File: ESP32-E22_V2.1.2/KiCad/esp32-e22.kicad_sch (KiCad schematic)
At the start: 46 parts, among them J1 Conn_01x02_Socket, J10 Conn_01x02_Socket, J11 Conn_01x04_Socket, J12 Conn_01x02_Socket, J3 Screw_Terminal_01x02, J4 Conn_01x04_Socket, J5 Conn_01x03_Socket, J6 Conn_01x04_Socket, J7 Conn_01x05_Socket, J8 SMA, J9 Conn_01x02_Socket, SW1 SW_Push, U1 ESP32-DevKitC V4, U2 DM-OLED096-636, U3 E22-400M33S, U4 HW-613

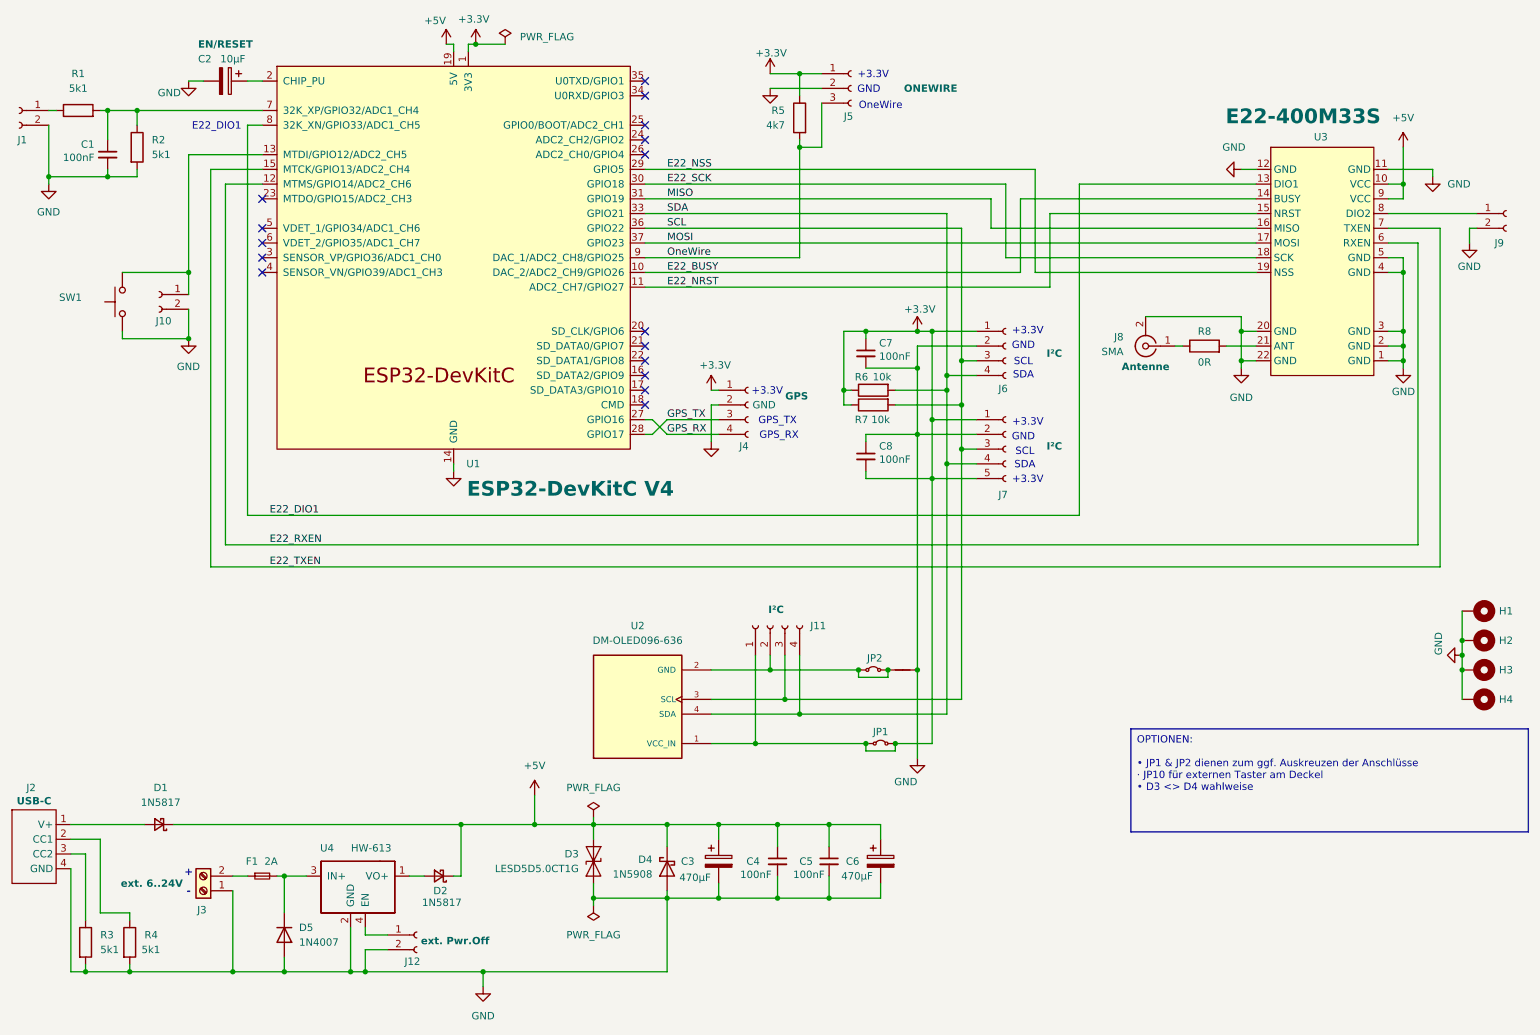
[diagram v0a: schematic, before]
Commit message: update
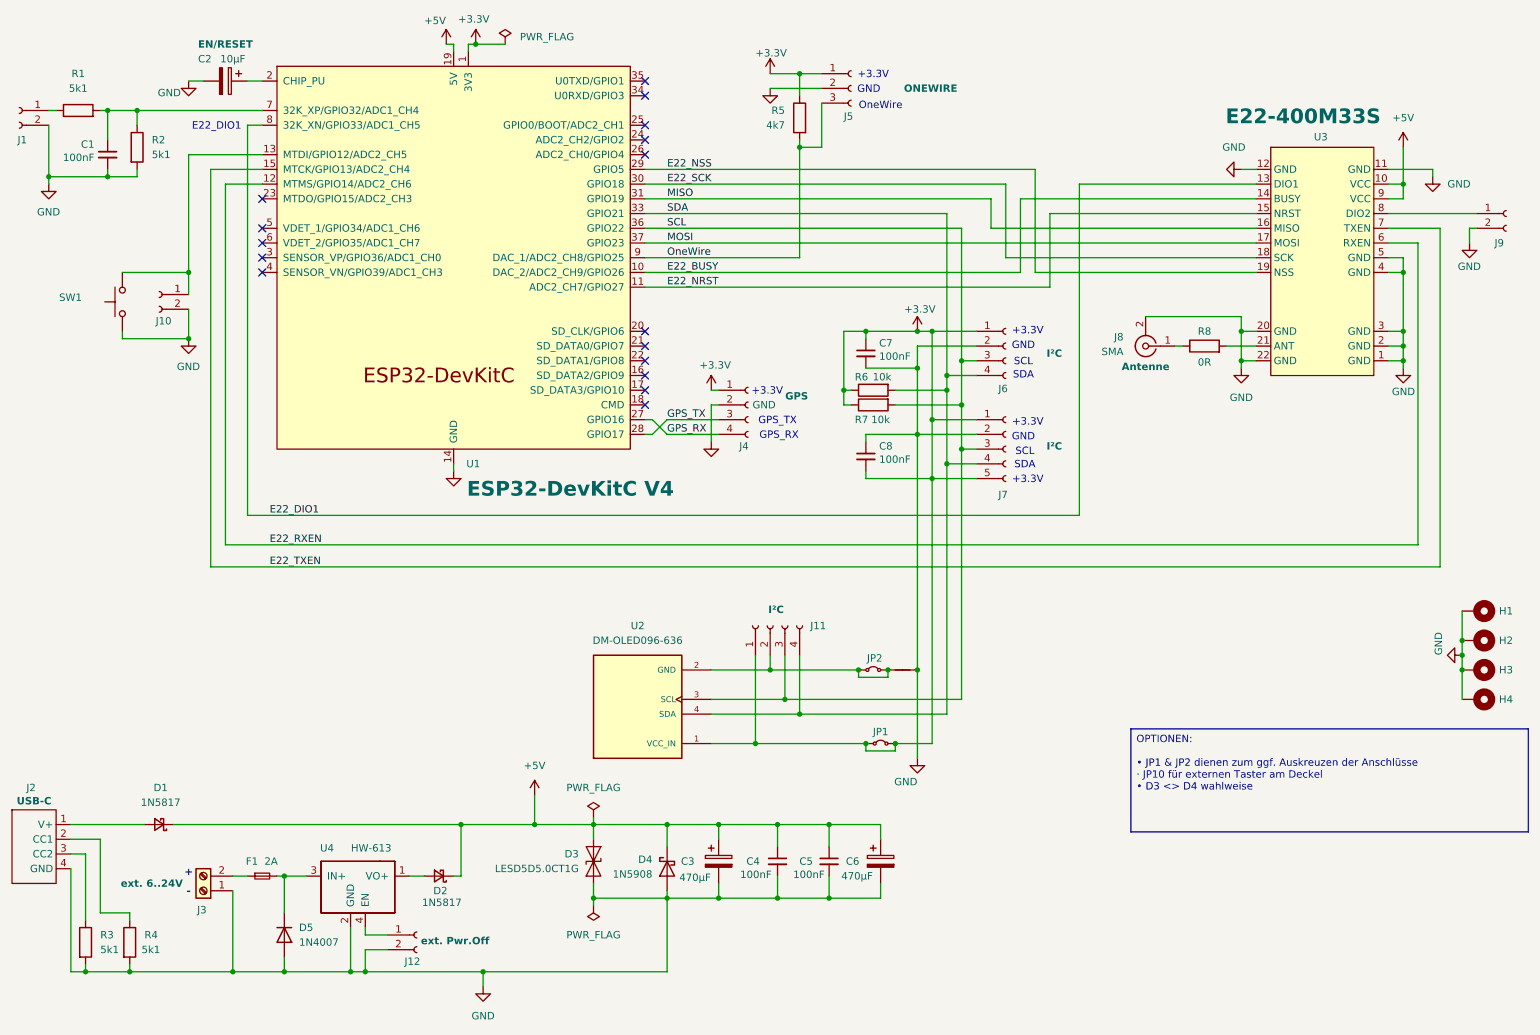
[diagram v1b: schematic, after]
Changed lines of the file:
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@@
 (kicad_sch
-	(version 20231120)
+	(version 20250114)
 	(generator "eeschema")
-	(generator_version "8.0")
+	(generator_version "9.0")
 	(paper "A4")
 	(title_block
@@
 		(company "OE3WAS")
 	)
+	(text "GND"
+		(exclude_from_sim no)
+		(at 193.548 94.488 0)
+		(effects
+			(font
+				(size 1.27 1.27)
+			)
+		)
+	)
+	(text "SCL"
+		(exclude_from_sim no)
+		(at 193.548 81.534 0)
+		(effects
+			(font
+				(size 1.27 1.27)
+			)
+		)
+	)
+	(text "GND"
+		(exclude_from_sim no)
+		(at 193.548 78.74 0)
+		(effects
+			(font
+				(size 1.27 1.27)
+			)
+		)
+	)
+	(text "SCL"
+		(exclude_from_sim no)
+		(at 193.802 97.028 0)
+		(effects
+			(font
+				(size 1.27 1.27)
+			)
+		)
+	)
+	(text "+3.3V"
+		(exclude_from_sim no)
+		(at 149.352 86.614 0)
+		(effects
+			(font
+				(size 1.27 1.27)
+			)
+		)
+	)
+	(text "+3.3V"
+		(exclude_from_sim no)
+		(at 194.31 101.854 0)
+		(effects
+			(font
+				(size 1.27 1.27)
+			)
+		)
+	)
+	(text "GND"
+		(exclude_from_sim no)
+		(at 166.878 34.544 0)
+		(effects
+			(font
+				(size 1.27 1.27)
+			)
+		)
+	)
+	(text "-"
+		(exclude_from_sim no)
+		(at 49.53 172.974 0)
+		(effects
+			(font
+				(size 1.27 1.27)
+				(thickness 0.254)
+				(bold yes)
+			)
+		)
+	)
+	(text "GPS_TX"
+		(exclude_from_sim no)
+		(at 151.13 91.694 0)
+		(effects
+			(font
+				(size 1.27 1.27)
+			)
+		)
+	)
+	(text "OneWire"
+		(exclude_from_sim no)
+		(at 168.91 37.338 0)
+		(effects
+			(font
+				(size 1.27 1.27)
+			)
+		)
+	)
+	(text "SDA"
+		(exclude_from_sim no)
+		(at 193.802 99.314 0)
+		(effects
+			(font
+				(size 1.27 1.27)
+			)
+		)
+	)
+	(text "SDA"
+		(exclude_from_sim no)
+		(at 193.548 83.82 0)
+		(effects
+			(font
+				(size 1.27 1.27)
+			)
+		)
+	)
+	(text "+3.3V"
+		(exclude_from_sim no)
+		(at 194.31 76.2 0)
+		(effects
+			(font
+				(size 1.27 1.27)
+			)
+		)
+	)
+	(text "+"
+		(exclude_from_sim no)
+		(at 49.53 169.672 0)
+		(effects
+			(font
+				(size 1.27 1.27)
+				(thickness 0.254)
+				(bold yes)
+			)
+		)
+	)
+	(text "GPS_RX"
+		(exclude_from_sim no)
+		(at 151.384 94.234 0)
+		(effects
+			(font
+				(size 1.27 1.27)
+			)
+		)
+	)
+	(text "+3.3V"
+		(exclude_from_sim no)
+		(at 194.31 91.948 0)
+		(effects
+			(font
+				(size 1.27 1.27)
+			)
+		)
+	)
+	(text "E22_DIO1"
+		(exclude_from_sim no)
+		(at 54.356 40.894 0)
+		(effects
+			(font
+				(size 1.27 1.27)
+			)
+		)
+	)
+	(text "+3.3V"
+		(exclude_from_sim no)
+		(at 167.64 32.004 0)
+		(effects
+			(font
+				(size 1.27 1.27)
+			)
+		)
+	)
+	(text_box "OPTIONEN:\n\n• JP1 & JP2 dienen zum ggf. Auskreuzen der Anschlüsse\n· JP10 für externen Taster am Deckel\n• D3 <> D4 wahlweise\n\n"
+		(exclude_from_sim yes)
+		(at 212.09 144.78 0)
+		(size 68.58 17.78)
+		(margins 0.9525 0.9525 0.9525 0.9525)
+		(stroke
+			(width 0)
+			(type default)
+		)
+		(fill
+			(type none)
+		)
+		(effects
+			(font
+				(size 1.27 1.27)
+			)
+			(justify left top)
+		)
+	)
 	(junction
 		(at 166.37 76.2)
@@
 		)
 	)
-	(text_box "OPTIONEN:\n\n• JP1 & JP2 dienen zum ggf. Auskreuzen der Anschlüsse\n· JP10 für externen Taster am Deckel\n• D3 <> D4 wahlweise\n\n"
-		(exclude_from_sim yes)
-		(at 212.09 144.78 0)
-		(size 68.58 17.78)
-		(stroke
-			(width 0)
-			(type default)
-		)
-		(fill
-			(type none)
-		)
-		(effects
-			(font
-				(size 1.27 1.27)
-			)
-			(justify left top)
-		)
-	)
-	(text "GND"
-		(exclude_from_sim no)
-		(at 193.548 94.488 0)
-		(effects
-			(font
-				(size 1.27 1.27)
-			)
-		)
-	)
-	(text "SCL"
-		(exclude_from_sim no)
-		(at 193.548 81.534 0)
-		(effects
-			(font
-				(size 1.27 1.27)
-			)
-		)
-	)
-	(text "GND"
-		(exclude_from_sim no)
-		(at 193.548 78.74 0)
-		(effects
-			(font
-				(size 1.27 1.27)
-			)
-		)
-	)
-	(text "SCL"
-		(exclude_from_sim no)
-		(at 193.802 97.028 0)
-		(effects
-			(font
-				(size 1.27 1.27)
-			)
-		)
-	)
-	(text "+3.3V"
-		(exclude_from_sim no)
-		(at 149.352 86.614 0)
-		(effects
-			(font
-				(size 1.27 1.27)
-			)
-		)
-	)
-	(text "+3.3V"
-		(exclude_from_sim no)
-		(at 194.31 101.854 0)
-		(effects
-			(font
-				(size 1.27 1.27)
-			)
-		)
-	)
-	(text "GND"
-		(exclude_from_sim no)
-		(at 166.878 34.544 0)
-		(effects
-			(font
-				(size 1.27 1.27)
-			)
-		)
-	)
-	(text "-"
-		(exclude_from_sim no)
-		(at 49.53 172.974 0)
-		(effects
-			(font
-				(size 1.27 1.27)
-				(thickness 0.254)
-				(bold yes)
-			)
-		)
-	)
-	(text "GPS_TX"
-		(exclude_from_sim no)
-		(at 151.13 91.694 0)
-		(effects
-			(font
-				(size 1.27 1.27)
-			)
-		)
-	)
-	(text "OneWire"
-		(exclude_from_sim no)
-		(at 168.91 37.338 0)
-		(effects
-			(font
-				(size 1.27 1.27)
-			)
-		)
-	)
-	(text "SDA"
-		(exclude_from_sim no)
-		(at 193.802 99.314 0)
-		(effects
-			(font
-				(size 1.27 1.27)
-			)
-		)
-	)
-	(text "SDA"
-		(exclude_from_sim no)
-		(at 193.548 83.82 0)
-		(effects
-			(font
-				(size 1.27 1.27)
-			)
-		)
-	)
-	(text "+3.3V"
-		(exclude_from_sim no)
-		(at 194.31 76.2 0)
-		(effects
-			(font
-				(size 1.27 1.27)
-			)
-		)
-	)
-	(text "+"
-		(exclude_from_sim no)
-		(at 49.53 169.672 0)
-		(effects
-			(font
-				(size 1.27 1.27)
-				(thickness 0.254)
-				(bold yes)
-			)
-		)
-	)
-	(text "GPS_RX"
-		(exclude_from_sim no)
-		(at 151.384 94.234 0)
-		(effects
-			(font
-				(size 1.27 1.27)
-			)
-		)
-	)
-	(text "+3.3V"
-		(exclude_from_sim no)
-		(at 194.31 91.948 0)
-		(effects
-			(font
-				(size 1.27 1.27)
-			)
-		)
-	)
-	(text "E22_DIO1"
-		(exclude_from_sim no)
-		(at 54.356 40.894 0)
-		(effects
-			(font
-				(size 1.27 1.27)
-			)
-		)
-	)
-	(text "+3.3V"
-		(exclude_from_sim no)
-		(at 167.64 32.004 0)
-		(effects
-			(font
-				(size 1.27 1.27)
-			)
-		)
-	)
 	(label "E22_NRST"
 		(at 132.08 68.58 0)
-		(fields_autoplaced yes)
 		(effects
 			(font
@@
 	(label "SCL"
 		(at 132.08 58.42 0)
-		(fields_autoplaced yes)
 		(effects
 			(font
@@
 	(label "E22_BUSY"
 		(at 132.08 66.04 0)
-		(fields_autoplaced yes)
 		(effects
 			(font
@@
 	(label "GPS_TX"
 		(at 132.08 91.44 0)
-		(fields_autoplaced yes)
 		(effects
 			(font
@@
 	(label "E22_SCK"
 		(at 132.08 50.8 0)
-		(fields_autoplaced yes)
 		(effects
 			(font
@@
 	(label "E22_RXEN"
 		(at 63.5 113.03 0)
-		(fields_autoplaced yes)
 		(effects
 			(font
@@
 	(label "E22_DIO1"
 		(at 63.5 107.95 0)
-		(fields_autoplaced yes)
 		(effects
 			(font
@@
 	(label "E22_TXEN"
 		(at 63.5 116.84 0)
-		(fields_autoplaced yes)
 		(effects
 			(font
@@
 	(label "GPS_RX"
 		(at 132.08 93.98 0)
-		(fields_autoplaced yes)
 		(effects
 			(font
@@
 	(label "MISO"
 		(at 132.08 53.34 0)
-		(fields_autoplaced yes)
 		(effects
 			(font
@@
 	(label "SDA"
 		(at 132.08 55.88 0)
-		(fields_autoplaced yes)
 		(effects
 			(font
@@
 	(label "MOSI"
 		(at 132.08 60.96 0)
-		(fields_autoplaced yes)
 		(effects
 			(font
@@
 	(label "E22_NSS"
 		(at 132.08 48.26 0)
-		(fields_autoplaced yes)
 		(effects
 			(font
@@
 	(label "OneWire"
 		(at 132.08 63.5 0)
-		(fields_autoplaced yes)
 		(effects
 			(font
@@
 		)
 	)
+	(embedded_fonts no)
 )
